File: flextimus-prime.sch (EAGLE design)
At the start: 41 parts, among them T1 2N2222, U1 STM32F042KXU, U2 IP4220CZ6, U3 MCP1802T-3302I/OT

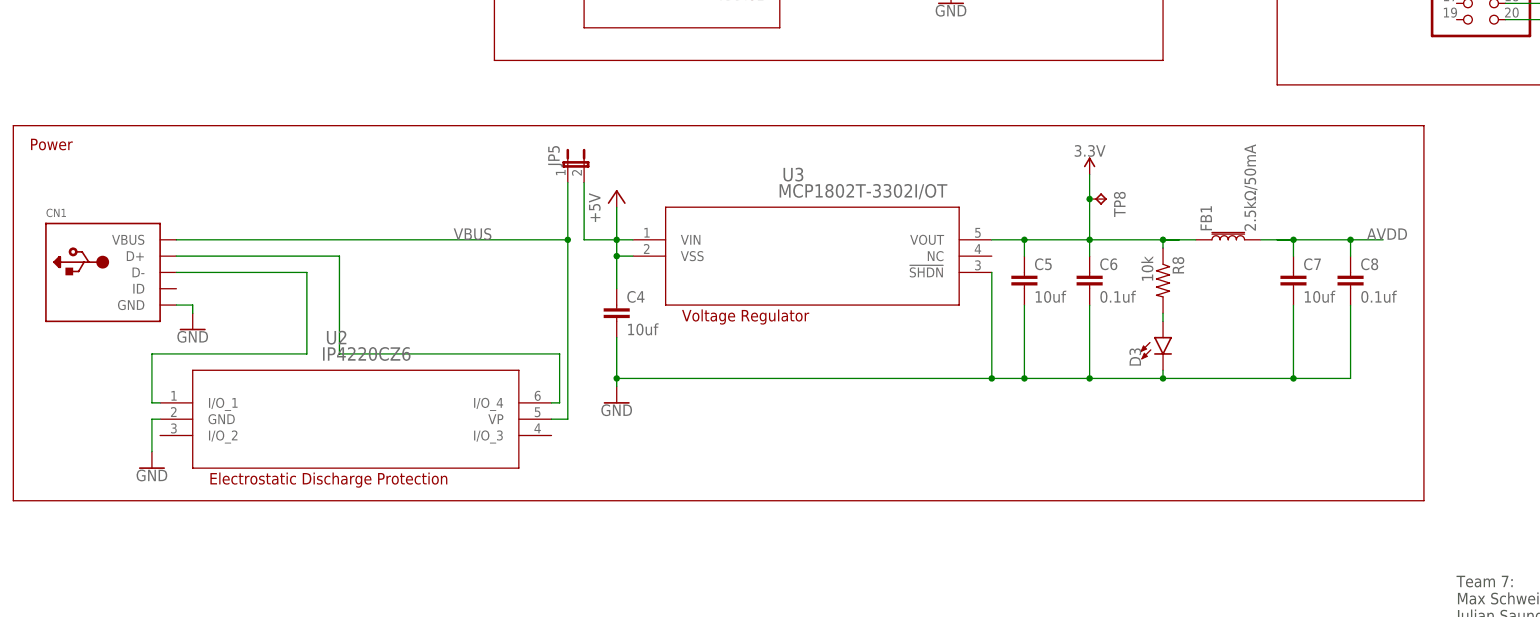
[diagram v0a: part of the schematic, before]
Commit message: better board, for real
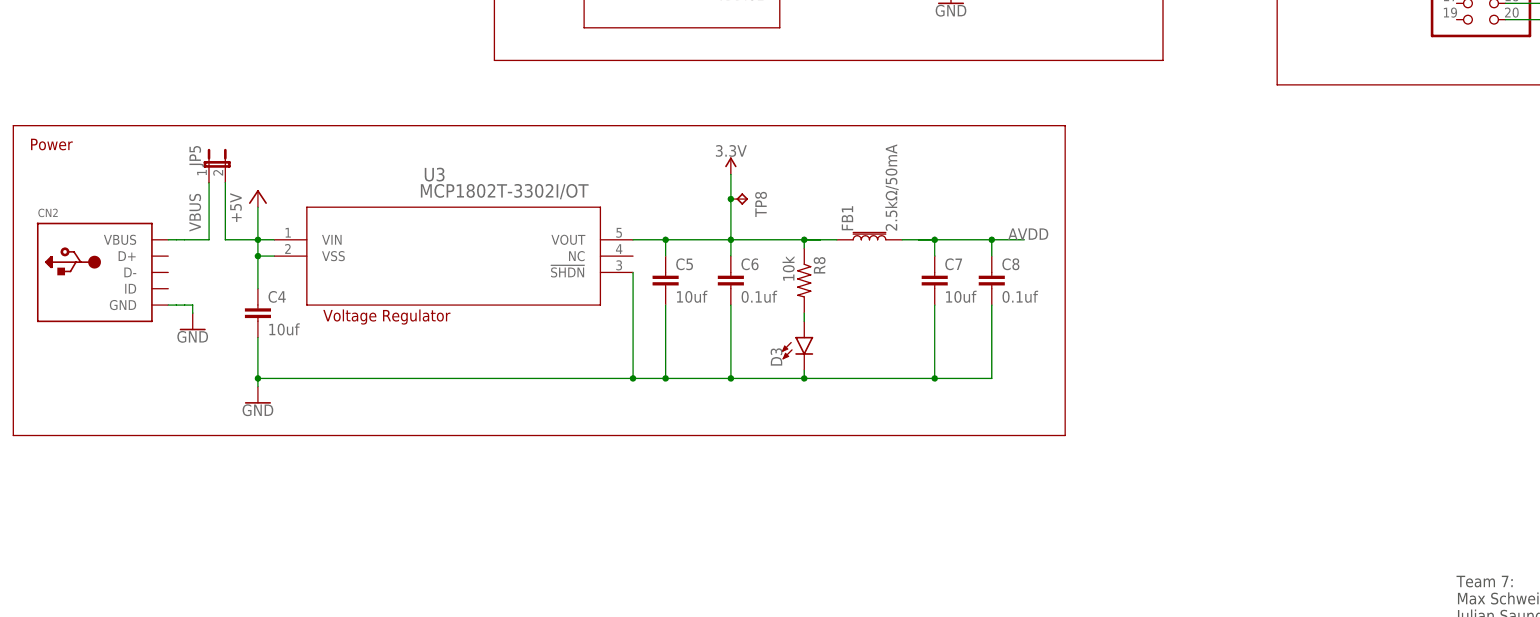
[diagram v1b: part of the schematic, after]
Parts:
- removed CN1: (no value), adafruit:USBMOLEX
- removed U2: IP4220CZ6, IP4220CZ6:IP4220CZ6
- added CN2: (no value), adafruit:USBMINIB
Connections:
- removed net USBM: CN1.D+, U2.I/O_4
- removed net USBP: CN1.D-, U2.I/O_1
- net GND: now also CN2.GND; no longer CN1.GND, U2.GND
- net VBUS: now also CN2.VBUS; no longer CN1.VBUS, U2.VP
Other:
- note removed: "Electrostatic Discharge Protection"
- moved on the sheet: C4, C5, C6, C7, C8, D3, FB1, JP5, R8, TP8, U3
